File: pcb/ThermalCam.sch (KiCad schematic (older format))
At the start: 39 parts, among them J1 USB_B_Mini, SW2 SW_Push, SW3 SW_Push, U1 AMS1117-3.3, U2 AMG8833, U4 ESP32-WROOM-32, U5 ILI9341-HLG-18, U6 Arducam_SPI, U7 ESP32_PROG

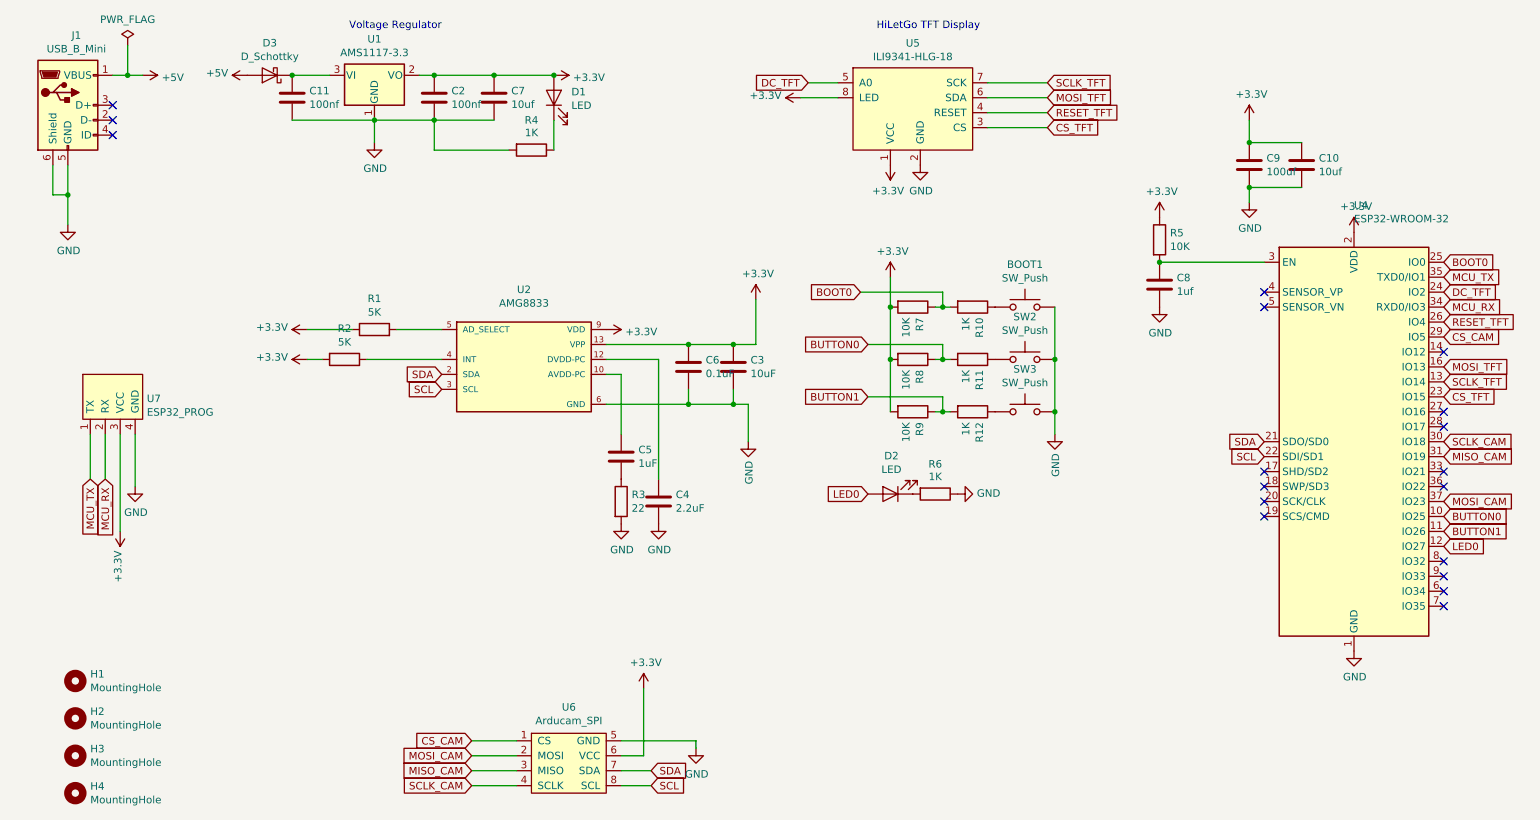
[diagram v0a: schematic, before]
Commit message: update
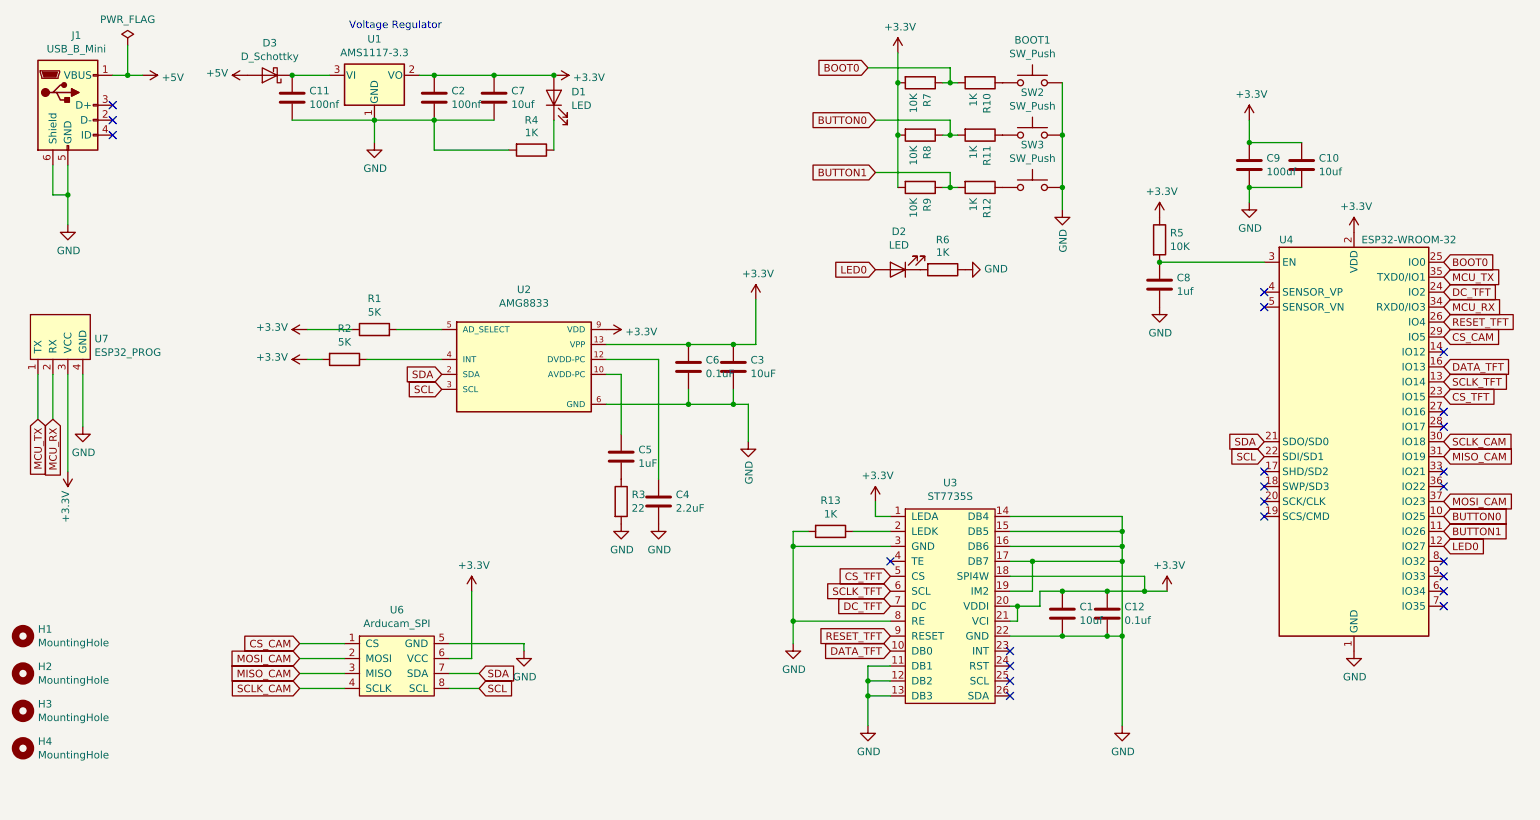
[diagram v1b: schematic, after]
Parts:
- removed U5: ILI9341-HLG-18, Connector_PinHeader_2.54mm:PinHeader_1x08_P2.54mm_Vertical, symbol ili9341-hlg-18:ILI9341-HLG-18
- added C1: 10uf, Capacitor_SMD:C_1206_3216Metric, symbol Device:C
- added C12: 0.1uf, Capacitor_SMD:C_1206_3216Metric, symbol Device:C
- added R13: 1K, Resistor_SMD:R_1206_3216Metric, symbol Device:R
- added U3: ST7735S, EastRising:ER-CON26HT-1, symbol EastRising:ER-TFT1.44-1
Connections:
- net +3V3: now also C1.1, C12.1, U3.1 (LEDA), U3.18 (SPI4W), U3.20 (VDDI), U3.21 (VCI)
- net CS_TFT: now also U3.5 (CS)
- net DC_TFT: now also U3.7 (DC)
- net GND: now also C1.2, C12.2, R13.2, U3.11 (DB1), U3.12 (DB2), U3.13 (DB3), U3.14 (DB4), U3.15 (DB5), U3.16 (DB6), U3.17 (DB7), U3.19 (IM2), U3.22 (GND), U3.3 (GND), U3.8 (RE)
- net RESET_TFT: now also U3.9 (RESET)
- net SCLK_TFT: now also U3.6 (SCL)
- net MOSI_TFT renamed DATA_TFT
- net DATA_TFT: now also U3.10 (DB0)
- new net: R13.1, U3.2 (LEDK)
- no-connect marks 18 -> 23
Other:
- note removed: "HiLetGo TFT Display"
- moved on the sheet: BOOT1, D2, H1, H2, H3, H4, R10, R11, R12, R6, R7, R8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
